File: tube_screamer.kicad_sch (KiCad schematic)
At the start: 38 parts, among them Q1 BC817, U1 TL072

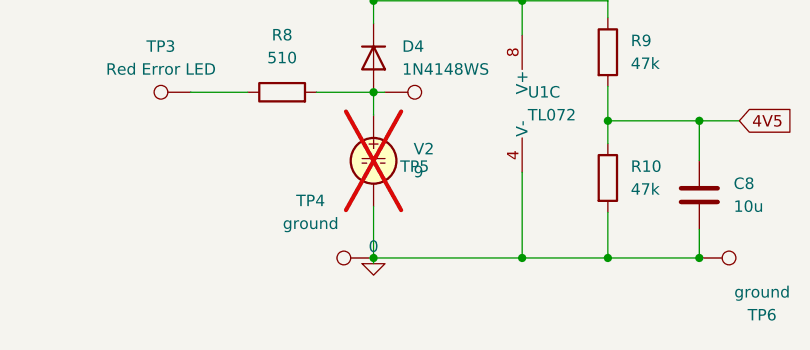
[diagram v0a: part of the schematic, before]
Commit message: PCB layout.
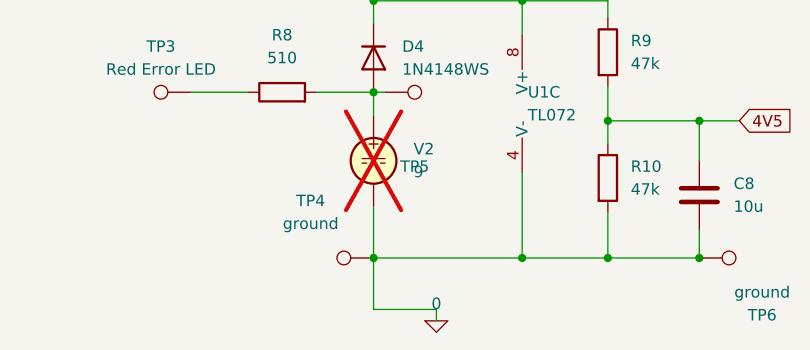
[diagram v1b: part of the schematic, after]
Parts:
- U1: footprint Package_SO:SOIC-8-1EP_3.9x4.9mm_P1.27mm_EP2.514x3.2mm -> Package_SO:SOIC-8_3.9x4.9mm_P1.27mm
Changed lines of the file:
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@@
 	(wire
 		(pts
-			(xy 85.725 178.435) (xy 85.725 179.07)
+			(xy 92.71 184.15) (xy 92.71 185.42)
 		)
 		(stroke
@@
 	(wire
 		(pts
+			(xy 85.725 184.15) (xy 85.725 178.435)
+		)
+		(stroke
+			(width 0)
+			(type default)
+		)
+	)
+	(wire
+		(pts
 			(xy 80.01 65.405) (xy 81.915 65.405)
 		)
@@
 	(wire
 		(pts
+			(xy 92.71 184.15) (xy 85.725 184.15)
+		)
+		(stroke
+			(width 0)
+			(type default)
+		)
+	)
+	(wire
+		(pts
 			(xy 121.92 80.01) (xy 121.285 80.01)
 		)
@@
 			)
 		)
-		(property "Footprint" "Package_SO:SOIC-8-1EP_3.9x4.9mm_P1.27mm_EP2.514x3.2mm"
+		(property "Footprint" "Package_SO:SOIC-8_3.9x4.9mm_P1.27mm"
 			(at 129.54 82.55 0)
 			(effects
@@
 			)
 		)
-		(property "Footprint" "Package_SO:SOIC-8-1EP_3.9x4.9mm_P1.27mm_EP2.514x3.2mm"
+		(property "Footprint" "Package_SO:SOIC-8_3.9x4.9mm_P1.27mm"
 			(at 104.775 161.29 0)
 			(effects
@@
 	(symbol
 		(lib_id "Simulation_SPICE:0")
-		(at 85.725 179.07 0)
+		(at 92.71 185.42 0)
 		(unit 1)
 		(exclude_from_sim no)
@@
 		(fields_autoplaced yes)
 		(property "Reference" "#GND04"
-			(at 85.725 181.61 0)
+			(at 92.71 187.96 0)
 			(effects
 				(font
@@
 		)
 		(property "Value" "0"
-			(at 85.725 177.165 0)
+			(at 92.71 183.515 0)
 			(effects
 				(font
@@
 		)
 		(property "Footprint" ""
-			(at 85.725 179.07 0)
+			(at 92.71 185.42 0)
 			(effects
 				(font
@@
 		)
 		(property "Datasheet" "~"
-			(at 85.725 179.07 0)
+			(at 92.71 185.42 0)
 			(effects
 				(font
@@
 		)
 		(property "Description" ""
-			(at 85.725 179.07 0)
+			(at 92.71 185.42 0)
 			(effects
 				(font
@@
 			)
 		)
-		(property "Footprint" "Package_SO:SOIC-8-1EP_3.9x4.9mm_P1.27mm_EP2.514x3.2mm"
+		(property "Footprint" "Package_SO:SOIC-8_3.9x4.9mm_P1.27mm"
 			(at 186.055 85.09 0)
 			(effects
